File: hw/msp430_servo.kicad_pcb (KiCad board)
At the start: 2 copper layers, 25.4 x 30.5 mm, 45 parts, among them IC1 MSP430G2553IPW20, IC2 L78L33ACUTR, P1 CONN_01X02, P10 CONN_01X03, P2 CONN_01X01, P3 CONN_01X03, P4 CONN_01X03, P5 CONN_01X02, P6 CONN_01X02, P7 CONN_01X02, P8 CONN_01X02, P9 CONN_01X03, Q1 BC817-40, Q2 BC817-40

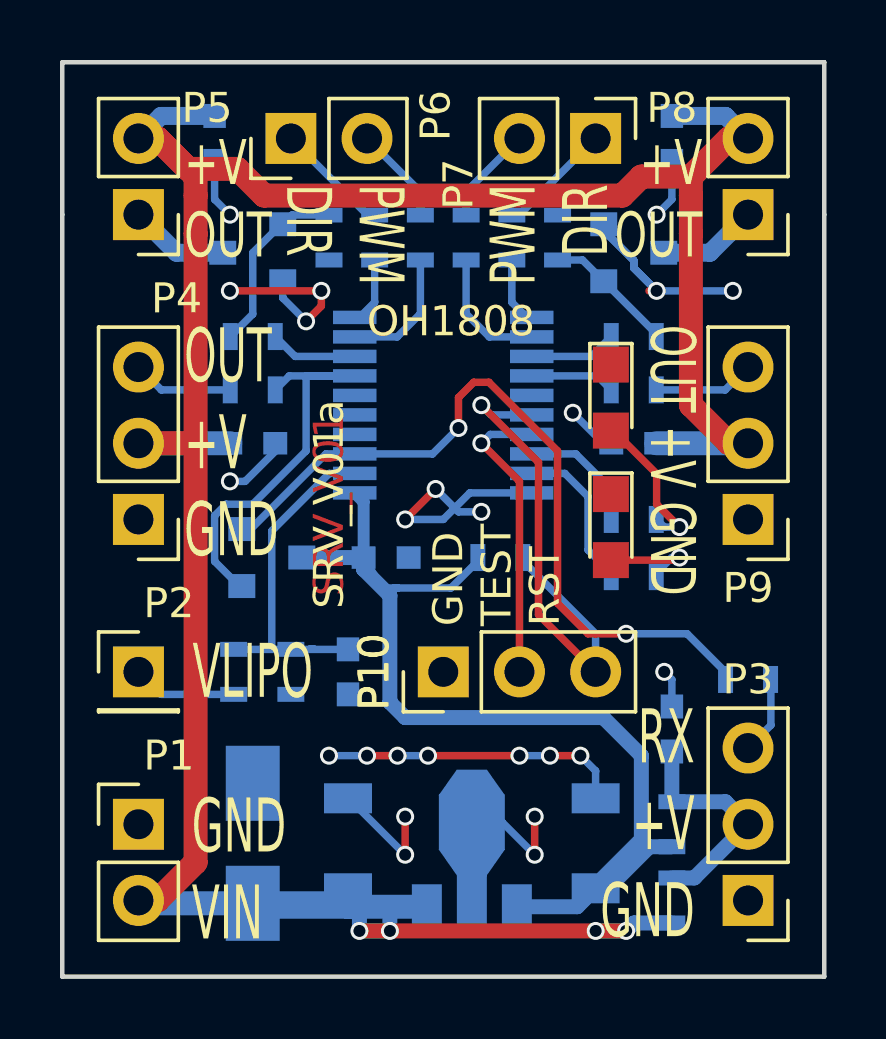
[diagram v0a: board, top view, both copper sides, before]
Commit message: v01a gerber data
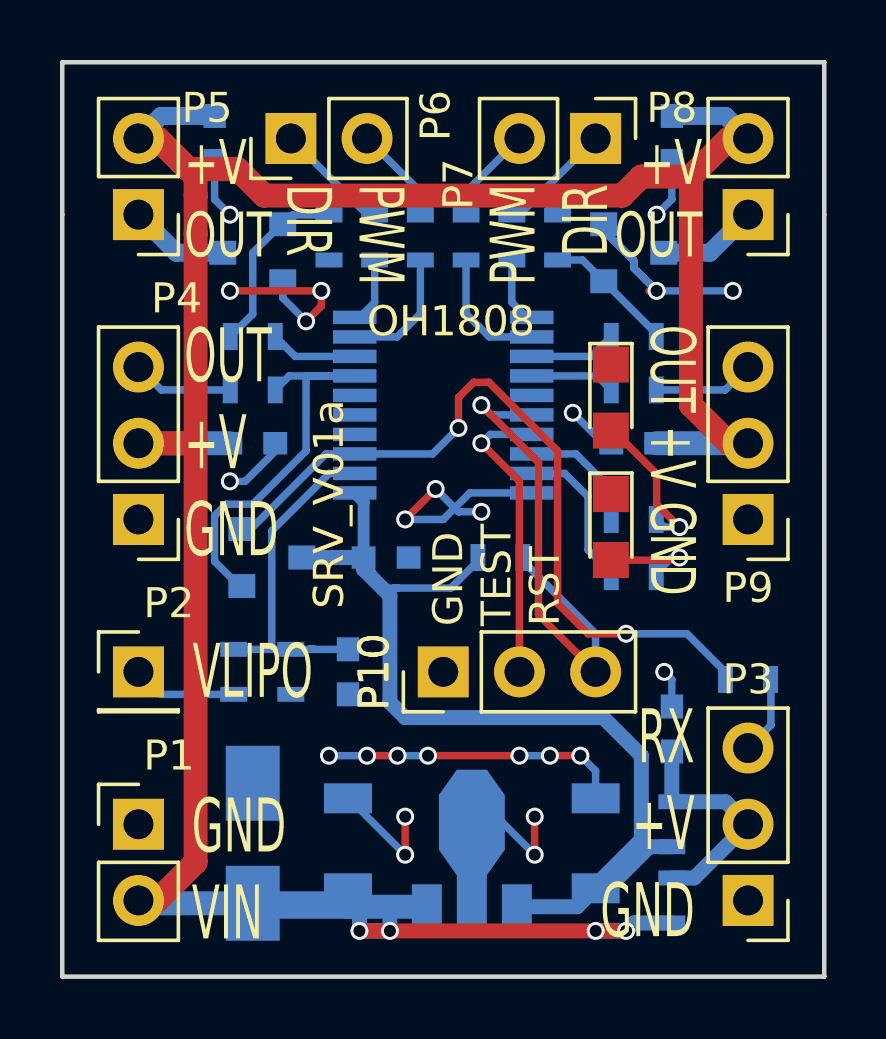
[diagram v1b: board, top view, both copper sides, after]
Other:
- board text removed: "SRV_V01"
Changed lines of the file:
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@@
     (visible_elements 7FFFFBFF)
     (pcbplotparams
-      (layerselection 0x010e0_80000001)
+      (layerselection 0x010e0_ffffffff)
       (usegerberextensions false)
       (usegerberattributes false)
@@
     (effects (font (size 1 1) (thickness 0.25)))
   )
-  (gr_text SRV_V01 (at 146.05 106.172 90) (layer F.Cu)
+  (gr_text SRV_V01a (at 146.05 106.172 90) (layer F.Cu)
     (effects (font (size 1 1) (thickness 0.25)))
   )
